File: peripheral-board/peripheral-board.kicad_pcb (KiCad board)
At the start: 2 copper layers, 165 x 100 mm, 248 parts, among them CON4001 BARREL_JACK, CON8001 SD_Card, J4001 53047-0510, J7001 FCR1295, J7002 53047-0310, P1001 Peripheral Bus, P1002 Power, Q4001 IRLML2244TRPbF, Q8001 BSS84LT1G, SW1001 Power, SW2001 1, SW2002 2, SW2003 3, SW2004 4, SW2005 5, SW2006 6, SW2007 7, SW2008 8, SW2009 9, SW2010 0, SW2011 +, SW2012 ´, SW2013 BKSP, SW2014 TROLL, SW2015 §, SW2016 UP, SW2017 RMB, SW2018 Q, SW2019 W, SW2020 E, SW2021 R, SW2022 T, SW2023 Y, SW2024 U, SW2025 I, SW2026 O, SW2027 P, SW2028 Å, SW2029 ¨, SW2030 RETURN, SW2031 ALT_GR, SW2032 <, SW2033 LEFT, SW2034 MMB, SW2035 A, SW2036 S, SW2037 D, SW2038 F, SW2039 G, SW2040 H, SW2041 J, SW2042 K, SW2043 L, SW2044 Ö, SW2045 Ä, SW2046 ', SW2047 ESC, SW2048 TAB, SW2049 ALT, SW2050 DOWN, SW2051 LMB, SW2052 SHIFT_L, SW2053 Z, SW2054 X, SW2055 C, SW2056 V, SW2057 B, SW2058 N, SW2059 M, SW2060 ,, SW2061 ., SW2062 -, SW2063 SHIFT_R, SW2064 FN_R, SW2065 SPACE, SW2066 FN_L, SW2067 RIGHT, SW2068 CTRL, SW2069 SPACE, U1001 ATTINY48-A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

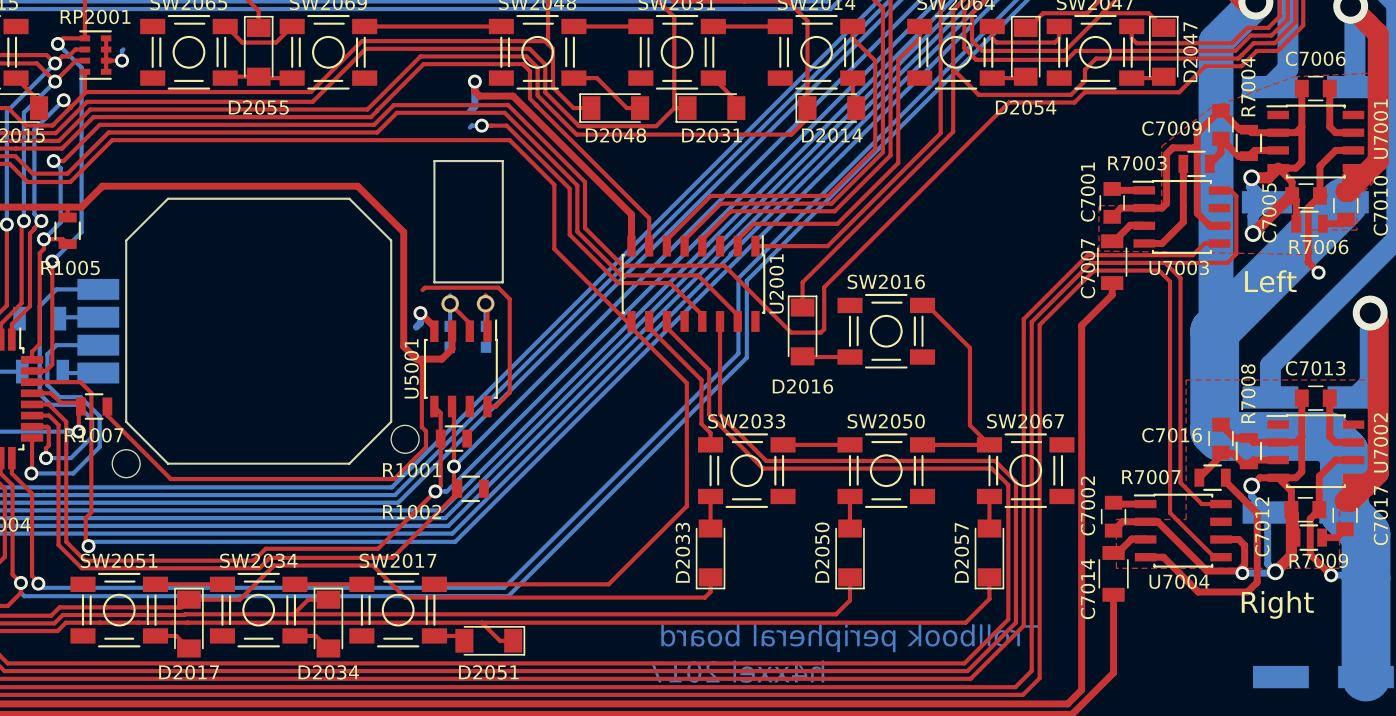
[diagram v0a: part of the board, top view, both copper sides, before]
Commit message: minor fixes to peripheral board
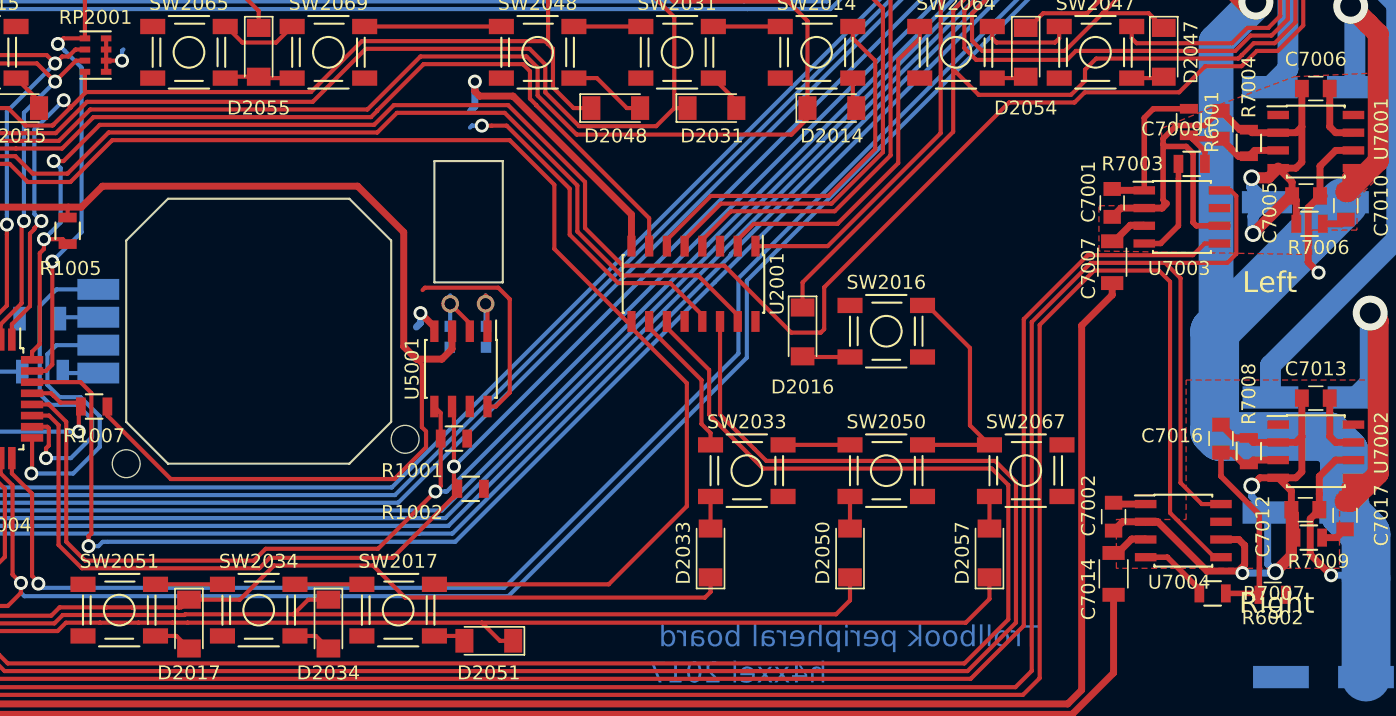
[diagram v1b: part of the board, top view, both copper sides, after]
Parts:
- added R6001: 10k, Resistors_SMD:R_0805, F.Cu at (234.2, 105.0)
- added R6002: 10k, Resistors_SMD:R_0805, F.Cu at (240.2, 138.9)
- L4002: value 10u -> 8u2
- R4012: value 270k -> 220k
- R4013: value 13.3k -> 12k
- moved R7007 8.30 mm to (235.9, 138.8), turned to 180 degrees
- moved R7003 0.35 mm to (234.4, 108.0)
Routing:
- net Net-(R7007-Pad2): track 17.8 -> 5.10 mm
- net Net-(C7016-Pad1): track 7.02 -> 18.6 mm
- net +3V3: track 267.7 -> 276.4 mm
- net GND: track 291.5 -> 295.2 mm
- net Net-(C7009-Pad1): track 6.92 -> 9.72 mm
